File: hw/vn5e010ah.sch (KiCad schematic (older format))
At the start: 3 parts, among them U1001 VN5E010AH

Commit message: working revision in FM_6.6.1
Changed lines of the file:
@@
 LIBS:wurth_elektronik_LED
 LIBS:power
-LIBS:elt21300_kicad
 LIBS:yageo
 LIBS:esb-cache
@@
 $Descr A4 11693 8268
 encoding utf-8
-Sheet 13 13
+Sheet 8 13
 Title ""
 Date ""
@@
 Text HLabel 3450 3200 0    60   Input ~ 0
 IN1
-Text HLabel 4350 3450 0    60   Output ~ 0
+Text HLabel 4350 3800 0    60   Output ~ 0
 SENSE1
 Wire Wire Line
@@
 	3450 3200 4900 3200
 Wire Wire Line
-	4350 3450 4600 3450
+	4350 3800 4600 3800
 $Comp
 L VDD #PWR602
@@
 AR Path="/5A01A445/59D7E637" Ref="#PWR702"  Part="1"
 AR Path="/5A01AB59/59D7E637" Ref="#PWR802"  Part="1"
-AR Path="/5A120DD2/59D7E637" Ref="#PWR602"  Part="1"
-AR Path="/5A12FF64/59D7E637" Ref="#PWR802"  Part="1"
-AR Path="/5A130D3E/59D7E637" Ref="#PWR902"  Part="1"
-AR Path="/5A1349CF/59D7E637" Ref="#PWR1002"  Part="1"
-AR Path="/5A1358B0/59D7E637" Ref="#PWR1102"  Part="1"
-AR Path="/5A13680F/59D7E637" Ref="#PWR1202"  Part="1"
-AR Path="/5A14370A/59D7E637" Ref="#PWR1302"  Part="1"
-F 0 "#PWR802" H 4600 2850 50  0001 C CNN
+AR Path="/5A120DD2/59D7E637" Ref="#PWR030"  Part="1"
+AR Path="/5A12FF64/59D7E637" Ref="#PWR036"  Part="1"
+AR Path="/5A130D3E/59D7E637" Ref="#PWR039"  Part="1"
+AR Path="/5A1349CF/59D7E637" Ref="#PWR042"  Part="1"
+AR Path="/5A1358B0/59D7E637" Ref="#PWR045"  Part="1"
+AR Path="/5A13680F/59D7E637" Ref="#PWR048"  Part="1"
+AR Path="/5A14370A/59D7E637" Ref="#PWR051"  Part="1"
+F 0 "#PWR051" H 4600 2850 50  0001 C CNN
 F 1 "VDD" H 4617 3173 50  0000 C CNN
 F 2 "" H 4600 3000 50  0000 C CNN
@@
 	4600 3000 4600 3100
 Wire Wire Line
-	4600 3450 4600 3300
+	4600 3800 4600 3300
 Connection ~ 4600 3300
 $Comp
@@
 AR Path="/5A01A445/5A014ACD" Ref="#PWR701"  Part="1"
 AR Path="/5A01AB59/5A014ACD" Ref="#PWR801"  Part="1"
-AR Path="/5A120DD2/5A014ACD" Ref="#PWR601"  Part="1"
-AR Path="/5A12FF64/5A014ACD" Ref="#PWR801"  Part="1"
-AR Path="/5A130D3E/5A014ACD" Ref="#PWR901"  Part="1"
-AR Path="/5A1349CF/5A014ACD" Ref="#PWR1001"  Part="1"
-AR Path="/5A1358B0/5A014ACD" Ref="#PWR1101"  Part="1"
-AR Path="/5A13680F/5A014ACD" Ref="#PWR1201"  Part="1"
-AR Path="/5A14370A/5A014ACD" Ref="#PWR1301"  Part="1"
-F 0 "#PWR801" H 3850 3350 50  0001 C CNN
+AR Path="/5A120DD2/5A014ACD" Ref="#PWR031"  Part="1"
+AR Path="/5A12FF64/5A014ACD" Ref="#PWR037"  Part="1"
+AR Path="/5A130D3E/5A014ACD" Ref="#PWR040"  Part="1"
+AR Path="/5A1349CF/5A014ACD" Ref="#PWR043"  Part="1"
+AR Path="/5A1358B0/5A014ACD" Ref="#PWR046"  Part="1"
+AR Path="/5A13680F/5A014ACD" Ref="#PWR049"  Part="1"
+AR Path="/5A14370A/5A014ACD" Ref="#PWR052"  Part="1"
+F 0 "#PWR052" H 3850 3350 50  0001 C CNN
 F 1 "GND" H 3855 3427 50  0000 C CNN
 F 2 "" H 3850 3600 50  0000 C CNN
@@
 F 2 "usevolt:HPAK" H 4950 4250 60  0001 C CNN
 F 3 "http://www.st.com/content/ccc/resource/technical/document/datasheet/1e/52/ef/e0/cc/90/4e/2e/CD00240716.pdf/files/CD00240716.pdf/jcr:content/translations/en.CD00240716.pdf" H 5050 4350 60  0001 C CNN
-F 4 "497-10505-2-ND" H 5450 4750 60  0001 C CNN "1st Source Part Number"
-F 5 "Digikey" H 5350 4650 60  0001 C CNN "1st Source"
-F 6 "STMicroelectronics" H 5150 4450 60  0001 C CNN "Manufacturer"
-F 7 "VN5E010AHTR-E" H 5250 4550 60  0001 C CNN "Manufacturer Part Number"
+F 4 "STMicroelectronics" H 5150 4450 60  0001 C CNN "Manufacturer"
+F 5 "VN5E010AHTR-E" H 5250 4550 60  0001 C CNN "Manufacturer Part Number"
+F 6 "Digikey" H 5350 4650 60  0001 C CNN "1st Source"
+F 7 "497-10505-2-ND" H 5450 4750 60  0001 C CNN "1st Source Part Number"
 	1    5300 3300
 	1    0    0    -1
 $EndComp
 $Comp
-L GND #PWR1003
+L GND #PWR044
 U 1 1 5A32CF90
 P 4800 3600
-AR Path="/5A1349CF/5A32CF90" Ref="#PWR1003"  Part="1"
-AR Path="/5A14370A/5A32CF90" Ref="#PWR1303"  Part="1"
-AR Path="/5A120DD2/5A32CF90" Ref="#PWR603"  Part="1"
-AR Path="/5A12FF64/5A32CF90" Ref="#PWR803"  Part="1"
-AR Path="/5A130D3E/5A32CF90" Ref="#PWR903"  Part="1"
-AR Path="/5A1358B0/5A32CF90" Ref="#PWR1103"  Part="1"
-AR Path="/5A13680F/5A32CF90" Ref="#PWR1203"  Part="1"
-F 0 "#PWR803" H 4800 3350 50  0001 C CNN
+AR Path="/5A1349CF/5A32CF90" Ref="#PWR044"  Part="1"
+AR Path="/5A14370A/5A32CF90" Ref="#PWR053"  Part="1"
+AR Path="/5A120DD2/5A32CF90" Ref="#PWR032"  Part="1"
+AR Path="/5A12FF64/5A32CF90" Ref="#PWR038"  Part="1"
+AR Path="/5A130D3E/5A32CF90" Ref="#PWR041"  Part="1"
+AR Path="/5A1358B0/5A32CF90" Ref="#PWR047"  Part="1"
+AR Path="/5A13680F/5A32CF90" Ref="#PWR050"  Part="1"
+F 0 "#PWR053" H 4800 3350 50  0001 C CNN
 F 1 "GND" H 4805 3427 50  0000 C CNN
 F 2 "" H 4800 3600 50  0000 C CNN

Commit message: starting to redraw the pcb as a smaller (icu enclosure)
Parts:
- R1001: symbol 390 -> yageo:390
- R502: symbol 1K -> yageo:1K
- U1001: symbol VN5E010AH -> usevolt:VN5E010AH
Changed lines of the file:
@@
-EESchema Schematic File Version 2
-LIBS:esb-rescue
-LIBS:kemet
-LIBS:usevolt
-LIBS:wurth_elektronik_LED
-LIBS:power
-LIBS:yageo
+EESchema Schematic File Version 4
 LIBS:esb-cache
 EELAYER 26 0
@@
 	4350 3800 4600 3800
 $Comp
-L VDD #PWR602
+L power:VDD #PWR602
 U 1 1 59D7E637
 P 4600 3000
@@
 Connection ~ 4600 3300
 $Comp
-L GND #PWR601
+L power:GND #PWR601
 U 1 1 5A014ACD
 P 3850 3600
@@
 	3850 3300 3850 3600
 $Comp
-L 1K R502
+L yageo:1K R502
 U 1 1 5A058D94
 P 3600 3350
@@
 Connection ~ 3850 3550
 $Comp
-L 390 R1001
+L yageo:390 R1001
 U 1 1 5A32CF0E
 P 4150 3300
@@
 $EndComp
 $Comp
-L VN5E010AH U1001
+L usevolt:VN5E010AH U1001
 U 1 1 5A32CF4A
 P 5300 3300
@@
 $EndComp
 $Comp
-L GND #PWR044
+L power:GND #PWR044
 U 1 1 5A32CF90
 P 4800 3600

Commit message: alternator fault disabled pump power limitation
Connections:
- wire segments 16 -> 21
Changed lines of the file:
@@
 $Descr A4 11693 8268
 encoding utf-8
-Sheet 8 13
+Sheet 6 14
 Title ""
 Date ""
@@
 SENSE1
 Wire Wire Line
-	4350 3300 4900 3300
+	4350 3300 4600 3300
 Wire Wire Line
 	3850 3300 4050 3300
 Wire Wire Line
-	3450 3200 4900 3200
+	3450 3200 3600 3200
 Wire Wire Line
 	4350 3800 4600 3800
@@
 AR Path="/5A13680F/59D7E637" Ref="#PWR048"  Part="1"
 AR Path="/5A14370A/59D7E637" Ref="#PWR051"  Part="1"
-F 0 "#PWR051" H 4600 2850 50  0001 C CNN
+F 0 "#PWR030" H 4600 2850 50  0001 C CNN
 F 1 "VDD" H 4617 3173 50  0000 C CNN
 F 2 "" H 4600 3000 50  0000 C CNN
@@
 	5700 3300 5700 3200
 Wire Wire Line
-	5600 3200 6200 3200
+	5600 3200 5700 3200
 Connection ~ 5700 3200
 Wire Wire Line
@@
 AR Path="/5A13680F/5A014ACD" Ref="#PWR049"  Part="1"
 AR Path="/5A14370A/5A014ACD" Ref="#PWR052"  Part="1"
-F 0 "#PWR052" H 3850 3350 50  0001 C CNN
+F 0 "#PWR031" H 3850 3350 50  0001 C CNN
 F 1 "GND" H 3855 3427 50  0000 C CNN
 F 2 "" H 3850 3600 50  0000 C CNN
@@
 $EndComp
 Wire Wire Line
-	3850 3300 3850 3600
+	3850 3300 3850 3550
 $Comp
 L yageo:1K R502
@@
 AR Path="/5A13680F/5A058D94" Ref="R1502"  Part="1"
 AR Path="/5A14370A/5A058D94" Ref="R1602"  Part="1"
-F 0 "R801" V 3608 3408 45  0000 L CNN
+F 0 "R901" V 3608 3408 45  0000 L CNN
 F 1 "1K" V 3692 3408 45  0000 L CNN
 F 2 "yageo:0603" H 3630 3500 20  0001 C CNN
@@
 AR Path="/5A1358B0/5A32CF0E" Ref="R1101"  Part="1"
 AR Path="/5A13680F/5A32CF0E" Ref="R1202"  Part="1"
-F 0 "R802" H 4200 3484 45  0000 C CNN
+F 0 "R601" H 4200 3484 45  0000 C CNN
 F 1 "390" H 4200 3400 45  0000 C CNN
 F 2 "yageo:0603" H 4180 3450 20  0001 C CNN
@@
 AR Path="/5A1358B0/5A32CF4A" Ref="U1101"  Part="1"
 AR Path="/5A13680F/5A32CF4A" Ref="U1201"  Part="1"
-F 0 "U801" H 5250 3747 60  0000 C CNN
+F 0 "U601" H 5250 3747 60  0000 C CNN
 F 1 "VN5E010AH" H 5250 3641 60  0000 C CNN
 F 2 "usevolt:HPAK" H 4950 4250 60  0001 C CNN
@@
 AR Path="/5A1358B0/5A32CF90" Ref="#PWR047"  Part="1"
 AR Path="/5A13680F/5A32CF90" Ref="#PWR050"  Part="1"
-F 0 "#PWR053" H 4800 3350 50  0001 C CNN
+F 0 "#PWR032" H 4800 3350 50  0001 C CNN
 F 1 "GND" H 4805 3427 50  0000 C CNN
 F 2 "" H 4800 3600 50  0000 C CNN
@@
 $EndComp
 Wire Wire Line
-	4800 3400 4800 3600
+	4800 3400 4800 3500
 Wire Wire Line
 	4800 3500 4900 3500
@@
 	4900 3400 4800 3400
 Connection ~ 4800 3500
+Wire Wire Line
+	5700 3200 6200 3200
+Wire Wire Line
+	4600 3300 4900 3300
+Wire Wire Line
+	3600 3200 4900 3200
+Wire Wire Line
+	3850 3550 3850 3600
+Wire Wire Line
+	4800 3500 4800 3600
 $EndSCHEMATC

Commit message: drawing new version of esb, not finished
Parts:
- removed R1001: 390, yageo:0603, symbol yageo:390
- added D1201: DIODE_RS07J-GS18, usevolt:DO219AB, symbol usevolt:DIODE_RS07J-GS18
- added R709: 1K, yageo:0603, symbol yageo:1K
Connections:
- net labels added: +3V3
- wire segments 21 -> 26
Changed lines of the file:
@@
 $Descr A4 11693 8268
 encoding utf-8
-Sheet 6 14
+Sheet 12 13
 Title ""
 Date ""
@@
 SENSE1
 Wire Wire Line
-	4350 3300 4600 3300
+	4350 3300 4450 3300
 Wire Wire Line
 	3850 3300 4050 3300
@@
 AR Path="/5A13680F/59D7E637" Ref="#PWR048"  Part="1"
 AR Path="/5A14370A/59D7E637" Ref="#PWR051"  Part="1"
-F 0 "#PWR030" H 4600 2850 50  0001 C CNN
+F 0 "#PWR051" H 4600 2850 50  0001 C CNN
 F 1 "VDD" H 4617 3173 50  0000 C CNN
 F 2 "" H 4600 3000 50  0000 C CNN
@@
 AR Path="/5A13680F/5A014ACD" Ref="#PWR049"  Part="1"
 AR Path="/5A14370A/5A014ACD" Ref="#PWR052"  Part="1"
-F 0 "#PWR031" H 3850 3350 50  0001 C CNN
+F 0 "#PWR052" H 3850 3350 50  0001 C CNN
 F 1 "GND" H 3855 3427 50  0000 C CNN
 F 2 "" H 3850 3600 50  0000 C CNN
@@
 AR Path="/5A13680F/5A058D94" Ref="R1502"  Part="1"
 AR Path="/5A14370A/5A058D94" Ref="R1602"  Part="1"
-F 0 "R901" V 3608 3408 45  0000 L CNN
+F 0 "R1602" V 3608 3408 45  0000 L CNN
 F 1 "1K" V 3692 3408 45  0000 L CNN
 F 2 "yageo:0603" H 3630 3500 20  0001 C CNN
@@
 	3600 3550 3850 3550
 Connection ~ 3850 3550
-$Comp
-L yageo:390 R1001
-U 1 1 5A32CF0E
-P 4150 3300
-AR Path="/5A1349CF/5A32CF0E" Ref="R1001"  Part="1"
-AR Path="/5A14370A/5A32CF0E" Ref="R1302"  Part="1"
-AR Path="/5A120DD2/5A32CF0E" Ref="R601"  Part="1"
-AR Path="/5A12FF64/5A32CF0E" Ref="R802"  Part="1"
-AR Path="/5A130D3E/5A32CF0E" Ref="R902"  Part="1"
-AR Path="/5A1358B0/5A32CF0E" Ref="R1101"  Part="1"
-AR Path="/5A13680F/5A32CF0E" Ref="R1202"  Part="1"
-F 0 "R601" H 4200 3484 45  0000 C CNN
-F 1 "390" H 4200 3400 45  0000 C CNN
-F 2 "yageo:0603" H 4180 3450 20  0001 C CNN
-F 3 "" H 4119 3339 60  0001 C CNN
-F 4 "" H 4519 3739 60  0001 C CNN "1st Source Part Number"
-F 5 "Digikey" H 4419 3639 60  0001 C CNN "1st Source"
-F 6 "RC0603FR-07390RL" H 4319 3539 60  0001 C CNN "Manufacturer Part Number"
-F 7 "YAGEO" H 4219 3439 60  0001 C CNN "Manufacturer"
-	1    4150 3300
-	1    0    0    -1
-$EndComp
 $Comp
 L usevolt:VN5E010AH U1001
@@
 AR Path="/5A1358B0/5A32CF4A" Ref="U1101"  Part="1"
 AR Path="/5A13680F/5A32CF4A" Ref="U1201"  Part="1"
-F 0 "U601" H 5250 3747 60  0000 C CNN
+F 0 "U1301" H 5250 3747 60  0000 C CNN
 F 1 "VN5E010AH" H 5250 3641 60  0000 C CNN
 F 2 "usevolt:HPAK" H 4950 4250 60  0001 C CNN
@@
 AR Path="/5A1358B0/5A32CF90" Ref="#PWR047"  Part="1"
 AR Path="/5A13680F/5A32CF90" Ref="#PWR050"  Part="1"
-F 0 "#PWR032" H 4800 3350 50  0001 C CNN
+F 0 "#PWR053" H 4800 3350 50  0001 C CNN
 F 1 "GND" H 4805 3427 50  0000 C CNN
 F 2 "" H 4800 3600 50  0000 C CNN
@@
 Wire Wire Line
 	4800 3500 4800 3600
+$Comp
+L yageo:1K R?
+U 1 1 5B23824A
+P 4250 3300
+AR Path="/5A01611C/5B23824A" Ref="R?"  Part="1"
+AR Path="/5A019746/5B23824A" Ref="R?"  Part="1"
+AR Path="/5A01A445/5B23824A" Ref="R?"  Part="1"
+AR Path="/5A01AB59/5B23824A" Ref="R?"  Part="1"
+AR Path="/5A120DD2/5B23824A" Ref="R?"  Part="1"
+AR Path="/5A12FF64/5B23824A" Ref="R709"  Part="1"
+AR Path="/5A130D3E/5B23824A" Ref="R802"  Part="1"
+AR Path="/5A1349CF/5B23824A" Ref="R901"  Part="1"
+AR Path="/5A1358B0/5B23824A" Ref="R1001"  Part="1"
+AR Path="/5A13680F/5B23824A" Ref="R1101"  Part="1"
+AR Path="/5A14370A/5B23824A" Ref="R1202"  Part="1"
+F 0 "R1202" V 4258 3358 45  0000 L CNN
+F 1 "1K" V 4342 3358 45  0000 L CNN
+F 2 "yageo:0603" H 4280 3450 20  0001 C CNN
+F 3 "" H 4219 3339 60  0001 C CNN
+F 4 "" H 4619 3739 60  0001 C CNN "1st Source Part Number"
+F 5 "Digikey" H 4519 3639 60  0001 C CNN "1st Source"
+F 6 "RC0603FR-071KL" H 4419 3539 60  0001 C CNN "Manufacturer Part Number"
+F 7 "YAGEO" H 4319 3439 60  0001 C CNN "Manufacturer"
+	1    4250 3300
+	-1   0    0    1
+$EndComp
+$Comp
+L usevolt:DIODE_RS07J-GS18 D1201
+U 1 1 5B23844A
+P 4150 3000
+AR Path="/5A14370A/5B23844A" Ref="D1201"  Part="1"
+AR Path="/5A12FF64/5B23844A" Ref="D703"  Part="1"
+AR Path="/5A130D3E/5B23844A" Ref="D801"  Part="1"
+AR Path="/5A1349CF/5B23844A" Ref="D901"  Part="1"
+AR Path="/5A1358B0/5B23844A" Ref="D1001"  Part="1"
+AR Path="/5A13680F/5B23844A" Ref="D1101"  Part="1"
+F 0 "D1201" H 4100 2860 45  0000 C CNN
+F 1 "DIODE_RS07J-GS18" H 4170 2940 45  0001 L BNN
+F 2 "usevolt:DO219AB" H 4180 3150 20  0001 C CNN
+F 3 "http://www.vishay.com/docs/85742/rs07b.pdf" H 4170 3020 60  0001 C CNN
+F 4 "1864882" H 4770 3620 60  0001 C CNN "2nd Source Part Number"
+F 5 "Digi-Key" H 4470 3320 60  0001 C CNN "1st Source"
+F 6 "Farnell" H 4670 3520 60  0001 C CNN "2nd Source"
+F 7 "RS07J-GS18" H 4370 3220 60  0001 C CNN "Manufacturer Part Number"
+F 8 "RS07J-GS18-ND" H 4570 3420 60  0001 C CNN "1st Source Part Number"
+F 9 "Vishay Semiconductor Diodes Division" H 4270 3120 60  0001 C CNN "Manufacturer"
+	1    4150 3000
+	-1   0    0    1
+$EndComp
+$Comp
+L power:+3V3 #PWR0107
+U 1 1 5B23856B
+P 3900 2850
+AR Path="/5A14370A/5B23856B" Ref="#PWR0107"  Part="1"
+AR Path="/5A12FF64/5B23856B" Ref="#PWR0102"  Part="1"
+AR Path="/5A130D3E/5B23856B" Ref="#PWR0103"  Part="1"
+AR Path="/5A1349CF/5B23856B" Ref="#PWR0104"  Part="1"
+AR Path="/5A1358B0/5B23856B" Ref="#PWR0105"  Part="1"
+AR Path="/5A13680F/5B23856B" Ref="#PWR0106"  Part="1"
+F 0 "#PWR0107" H 3900 2700 50  0001 C CNN
+F 1 "+3V3" H 3915 3023 50  0000 C CNN
+F 2 "" H 3900 2850 50  0000 C CNN
+F 3 "" H 3900 2850 50  0000 C CNN
+	1    3900 2850
+	1    0    0    -1
+$EndComp
+Wire Wire Line
+	3900 2850 3900 3000
+Wire Wire Line
+	3900 3000 4050 3000
+Wire Wire Line
+	4350 3000 4450 3000
+Wire Wire Line
+	4450 3000 4450 3300
+Connection ~ 4450 3300
+Wire Wire Line
+	4450 3300 4600 3300
 $EndSCHEMATC

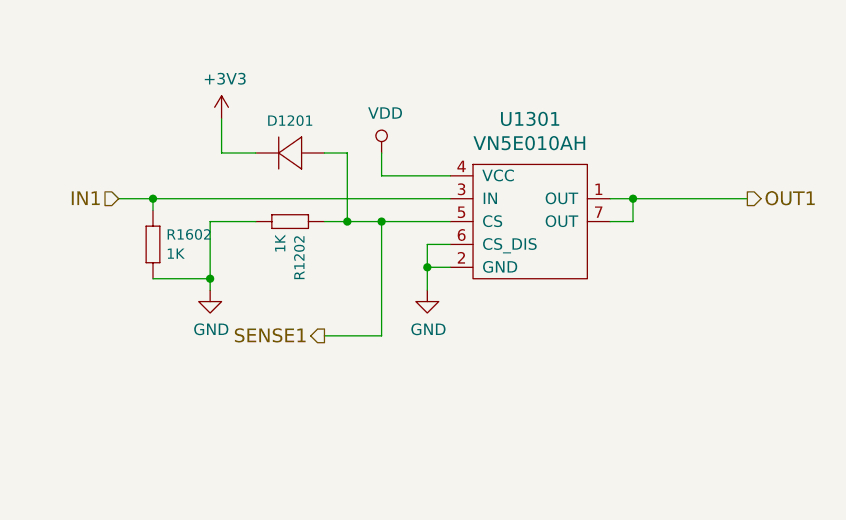
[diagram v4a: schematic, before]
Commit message: hw version 5.0.0, for hcu enclosure
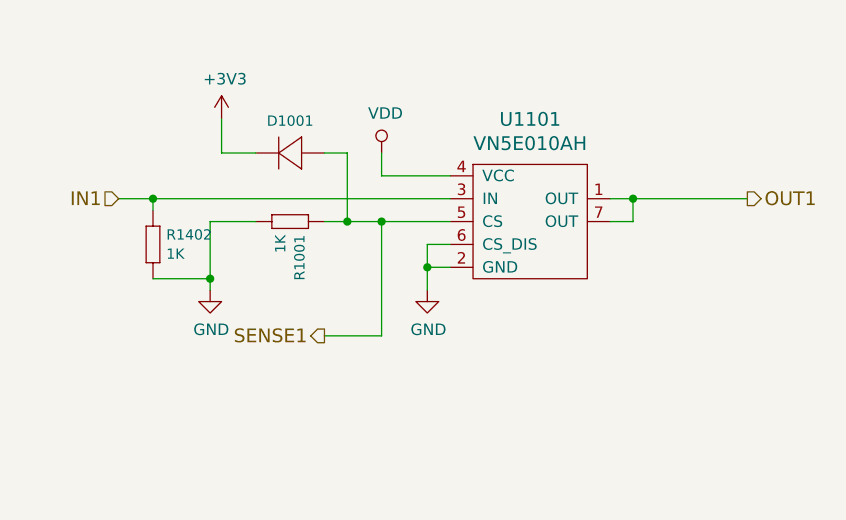
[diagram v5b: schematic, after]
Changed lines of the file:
@@
 $Descr A4 11693 8268
 encoding utf-8
-Sheet 12 13
+Sheet 7 12
 Title ""
 Date ""
@@
 AR Path="/5A13680F/59D7E637" Ref="#PWR048"  Part="1"
 AR Path="/5A14370A/59D7E637" Ref="#PWR051"  Part="1"
-F 0 "#PWR051" H 4600 2850 50  0001 C CNN
+F 0 "#PWR045" H 4600 2850 50  0001 C CNN
 F 1 "VDD" H 4617 3173 50  0000 C CNN
 F 2 "" H 4600 3000 50  0000 C CNN
@@
 AR Path="/5A13680F/5A014ACD" Ref="#PWR049"  Part="1"
 AR Path="/5A14370A/5A014ACD" Ref="#PWR052"  Part="1"
-F 0 "#PWR052" H 3850 3350 50  0001 C CNN
+F 0 "#PWR046" H 3850 3350 50  0001 C CNN
 F 1 "GND" H 3855 3427 50  0000 C CNN
 F 2 "" H 3850 3600 50  0000 C CNN
@@
 AR Path="/5A13680F/5A058D94" Ref="R1502"  Part="1"
 AR Path="/5A14370A/5A058D94" Ref="R1602"  Part="1"
-F 0 "R1602" V 3608 3408 45  0000 L CNN
+F 0 "R1402" V 3608 3408 45  0000 L CNN
 F 1 "1K" V 3692 3408 45  0000 L CNN
 F 2 "yageo:0603" H 3630 3500 20  0001 C CNN
@@
 AR Path="/5A1358B0/5A32CF4A" Ref="U1101"  Part="1"
 AR Path="/5A13680F/5A32CF4A" Ref="U1201"  Part="1"
-F 0 "U1301" H 5250 3747 60  0000 C CNN
+F 0 "U1101" H 5250 3747 60  0000 C CNN
 F 1 "VN5E010AH" H 5250 3641 60  0000 C CNN
 F 2 "usevolt:HPAK" H 4950 4250 60  0001 C CNN
@@
 AR Path="/5A1358B0/5A32CF90" Ref="#PWR047"  Part="1"
 AR Path="/5A13680F/5A32CF90" Ref="#PWR050"  Part="1"
-F 0 "#PWR053" H 4800 3350 50  0001 C CNN
+F 0 "#PWR047" H 4800 3350 50  0001 C CNN
 F 1 "GND" H 4805 3427 50  0000 C CNN
 F 2 "" H 4800 3600 50  0000 C CNN
@@
 AR Path="/5A13680F/5B23824A" Ref="R1101"  Part="1"
 AR Path="/5A14370A/5B23824A" Ref="R1202"  Part="1"
-F 0 "R1202" V 4258 3358 45  0000 L CNN
+F 0 "R1001" V 4258 3358 45  0000 L CNN
 F 1 "1K" V 4342 3358 45  0000 L CNN
 F 2 "yageo:0603" H 4280 3450 20  0001 C CNN
@@
 AR Path="/5A1358B0/5B23844A" Ref="D1001"  Part="1"
 AR Path="/5A13680F/5B23844A" Ref="D1101"  Part="1"
-F 0 "D1201" H 4100 2860 45  0000 C CNN
+F 0 "D1001" H 4100 2860 45  0000 C CNN
 F 1 "DIODE_RS07J-GS18" H 4170 2940 45  0001 L BNN
 F 2 "usevolt:DO219AB" H 4180 3150 20  0001 C CNN
@@
 AR Path="/5A1358B0/5B23856B" Ref="#PWR0105"  Part="1"
 AR Path="/5A13680F/5B23856B" Ref="#PWR0106"  Part="1"
-F 0 "#PWR0107" H 3900 2700 50  0001 C CNN
+F 0 "#PWR0105" H 3900 2700 50  0001 C CNN
 F 1 "+3V3" H 3915 3023 50  0000 C CNN
 F 2 "" H 3900 2850 50  0000 C CNN
